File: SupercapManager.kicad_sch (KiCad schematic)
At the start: 9 parts, among them J1 JST4_F, J2 XT30_F, J3 XT30_F, J4 XT30_F, J5 XT30_F, Q11 BSC059N04LS6, Q12 BSC059N04LS6

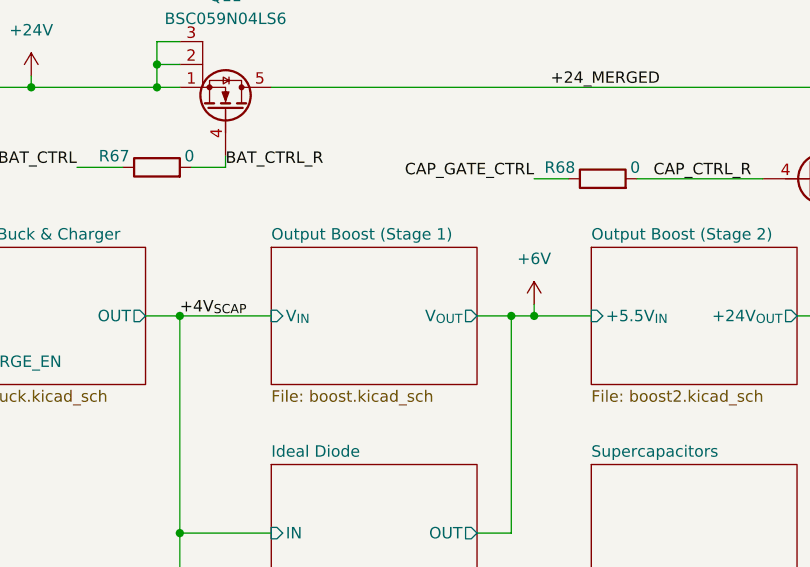
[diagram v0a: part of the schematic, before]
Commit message: Various schematic touchups
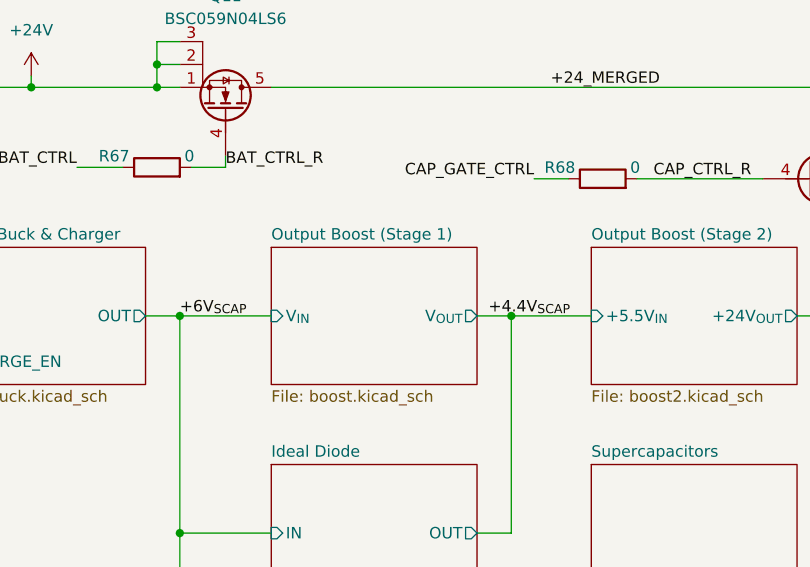
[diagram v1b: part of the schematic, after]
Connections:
- net +4V_{SCAP}: no longer J5.1 (Pin_1)
- new net +6V_{SCAP}: J5.1 (Pin_1)
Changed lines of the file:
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@@
-	)
-	(junction
-		(at 165.1 105.41)
-		(diameter 0)
-		(color 0 0 0 0)
 	)
 	(junction
@@
 	(wire
 		(pts
-			(xy 165.1 105.41) (xy 171.45 105.41)
+			(xy 162.56 105.41) (xy 171.45 105.41)
 		)
 		(stroke
@@
 	(wire
 		(pts
-			(xy 162.56 105.41) (xy 165.1 105.41)
-		)
-		(stroke
-			(width 0)
-			(type default)
-		)
-	)
-	(wire
-		(pts
 			(xy 95.25 105.41) (xy 100.33 105.41)
 		)
@@
 		(pts
 			(xy 198.12 85.09) (xy 198.12 80.01)
-		)
-		(stroke
-			(width 0)
-			(type default)
-		)
-	)
-	(wire
-		(pts
-			(xy 165.1 104.14) (xy 165.1 105.41)
 		)
 		(stroke
@@
 		)
 	)
+	(label "+4.4V_{SCAP}"
+		(at 160.02 105.41 0)
+		(effects
+			(font
+				(size 1.27 1.27)
+			)
+			(justify left bottom)
+		)
+	)
 	(label "+24_{MiniPC}"
 		(at 123.19 45.72 0)
@@
 		)
 	)
-	(label "+4V_{SCAP}"
+	(label "+6V_{SCAP}"
 		(at 125.73 105.41 0)
 		(effects
@@
 					(unit 1)
 				)
-			)
-		)
-	)
-	(symbol
-		(lib_id "power:+6V")
-		(at 165.1 104.14 0)
-		(unit 1)
-		(exclude_from_sim no)
-		(in_bom yes)
-		(on_board yes)
-		(dnp no)
-		(fields_autoplaced yes)
-		(property "Reference" "#PWR020"
-			(at 165.1 107.95 0)
-			(effects
-				(font
-					(size 1.27 1.27)
-				)
-				(hide yes)
-			)
-		)
-		(property "Value" "+6V"
-			(at 165.1 99.06 0)
-			(effects
-				(font
-					(size 1.27 1.27)
-				)
-			)
-		)
-		(property "Footprint" ""
-			(at 165.1 104.14 0)
-			(effects
-				(font
-					(size 1.27 1.27)
-				)
-				(hide yes)
-			)
-		)
-		(property "Datasheet" ""
-			(at 165.1 104.14 0)
-			(effects
-				(font
-					(size 1.27 1.27)
-				)
-				(hide yes)
-			)
-		)
-		(property "Description" "Power symbol creates a global label with name \"+6V\""
-			(at 165.1 104.14 0)
-			(effects
-				(font
-					(size 1.27 1.27)
-				)
-				(hide yes)
-			)
-		)
-		(pin "1"
-		)
-		(instances
-			(project ""
-				(path "/6197145b-e7d4-44cc-9d90-537b6501bf60"
-					(reference "#PWR020")
-					(unit 1)
-				)
